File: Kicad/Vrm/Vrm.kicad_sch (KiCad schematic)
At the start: 17 parts, among them J2 Screw_Terminal_01x02, J3 Screw_Terminal_01x02, J4 AVR-JTAG-10, Q1 2N3704, SW1 Switch, U1 STM32F091RCTx

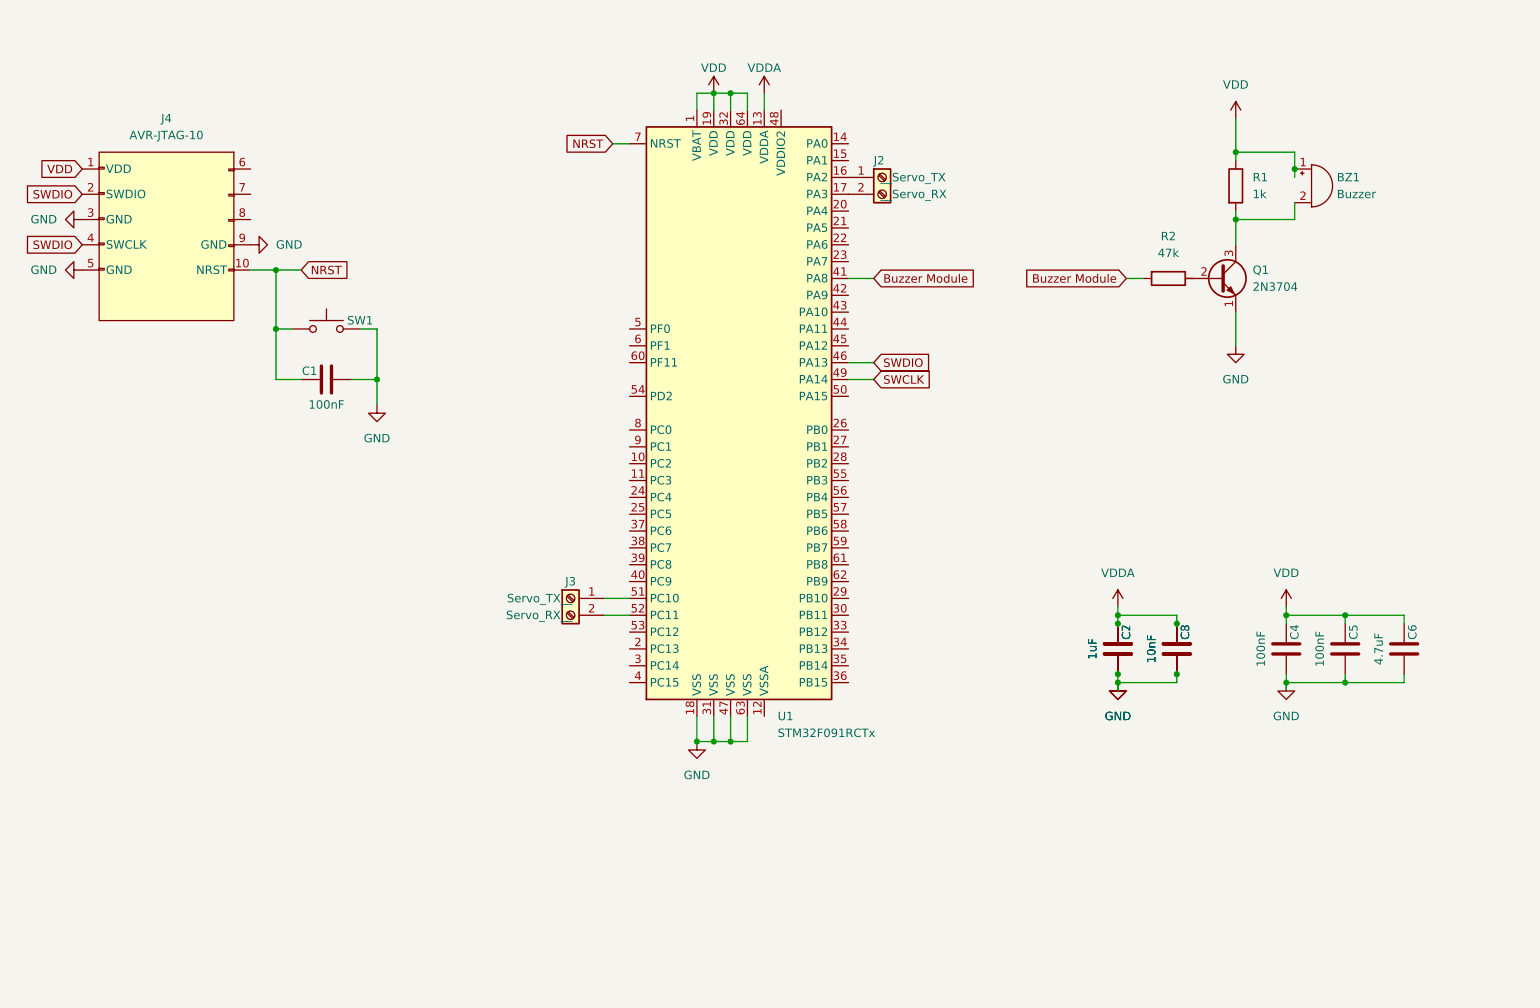
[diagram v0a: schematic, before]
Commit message: Updated schematic
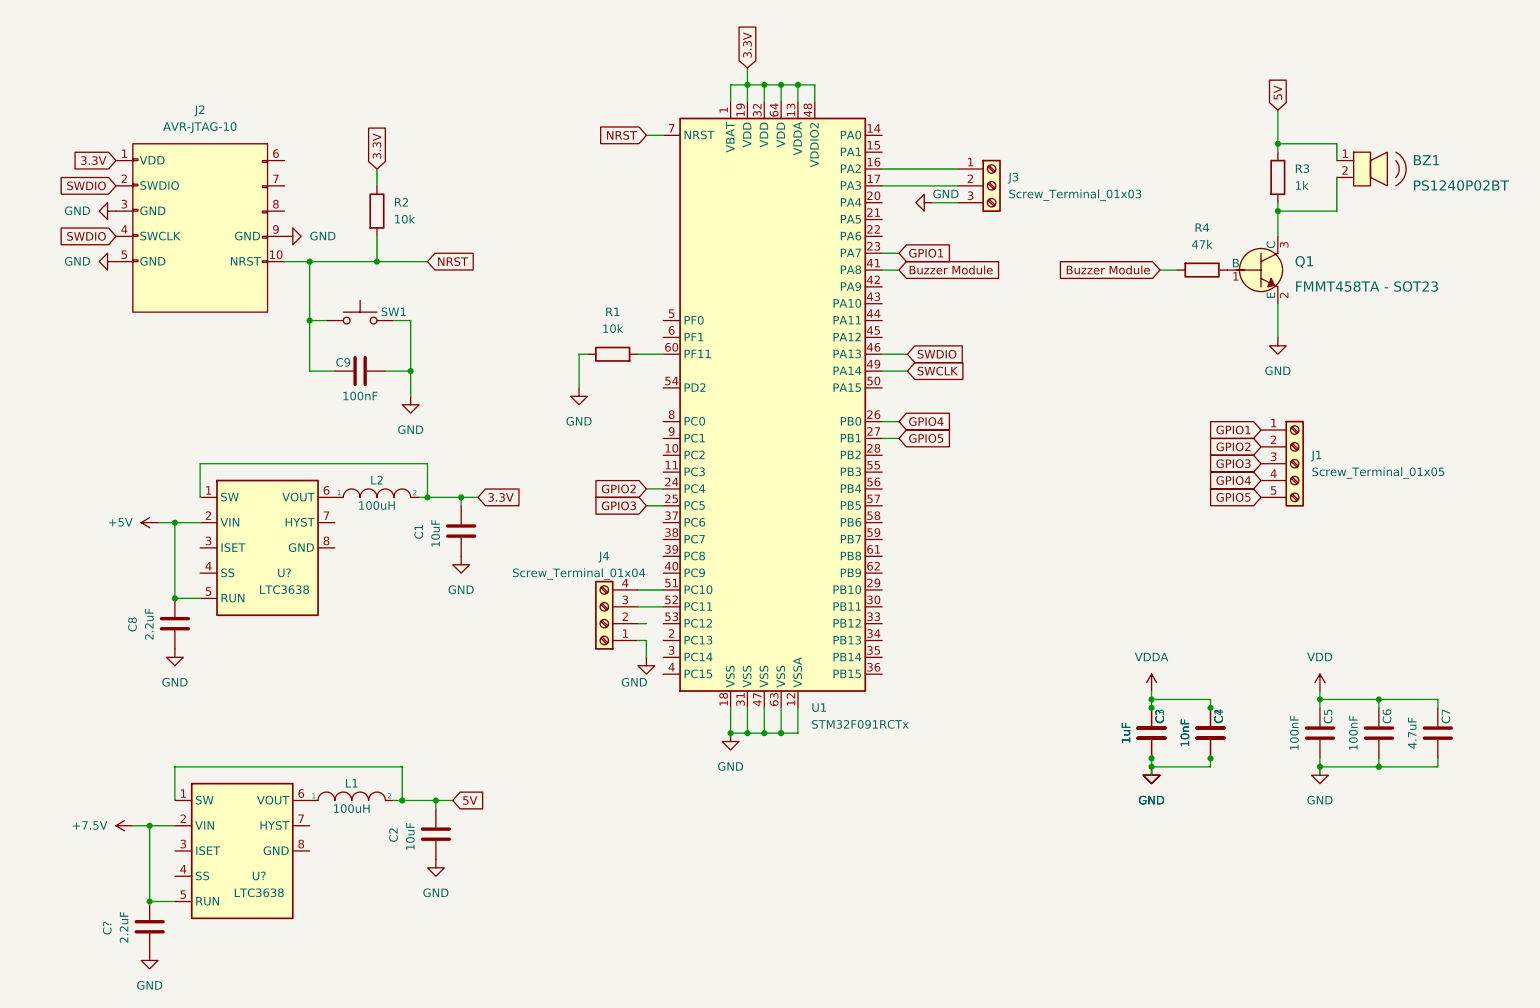
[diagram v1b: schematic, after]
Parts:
- removed BZ1: Buzzer, symbol Device:Buzzer
- removed J2, J3: Screw_Terminal_01x02, symbol Connector:Screw_Terminal_01x02
- removed J4: AVR-JTAG-10, symbol Connector:AVR-JTAG-10
- removed Q1: 2N3704, Package_TO_SOT_THT:TO-92_Inline, symbol Transistor_BJT:2N3904
- added BZ1: PS1240P02BT, digikey-footprints:Piezo_Transducer_THT_PS1240P02BT, symbol dk_Alarms-Buzzers-and-Sirens:PS1240P02BT
- added C9: 100nF, symbol Device:C
- added C?: 1uF, symbol Device:C
- added C?: 2.2uF, symbol Device:C
- added C?: 10nF, symbol Device:C
- added J1: Screw_Terminal_01x05, symbol Connector:Screw_Terminal_01x05
- added J2: AVR-JTAG-10, symbol Connector:AVR-JTAG-10
- added J3: Screw_Terminal_01x03, symbol Connector:Screw_Terminal_01x03
- added J4: Screw_Terminal_01x04, symbol Connector:Screw_Terminal_01x04
- added L1, L2: 100uH, symbol pspice:INDUCTOR
- added Q1: FMMT458TA - SOT23, digikey-footprints:SOT-23-3, symbol dk_Transistors-Bipolar-BJT-Single:FMMT458TA
- added R3: 1k, symbol Device:R
- added R4: 47k, symbol Device:R
- added U? (x2): LTC3638, Package_SO:Linear_MSOP-12-16-1EP_3x4mm_P0.5mm, symbol Regulator_Switching:LTC3638
- C1: value 100nF -> 10uF
- C2: value 1uF -> 10uF
- C3: value 10nF -> 1uF
- C4: value 100nF -> 10nF
- C6: value 4.7uF -> 100nF
- C7: value 1uF -> 4.7uF
- C8: value 10nF -> 2.2uF
- R1: value 1k -> 10k
- R2: value 47k -> 10k
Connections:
- net Buzzer Module: now also R4.2; no longer R2.2
- net GND: now also R1.1, U1.12 (VSSA), C9.2, C?.2, C?.2, C?.2, J2.3 (GND), J2.5 (GND), J2.9 (GND), J3.3 (Pin_3), J4.1 (Pin_1), Q1.2 (E)
- net NRST: now also R2.2, C9.1, J2.10 (NRST); no longer C1.1
- net SWDIO: now also J2.2 (SWDIO), J2.4 (SWCLK)
- net VDD: now also C7.1; no longer C4.1, R1.1, U1.1 (VBAT), U1.19 (VDD), U1.32 (VDD), U1.64 (VDD)
- net VDDA: now also C4.1, C?.1, C?.1; no longer C2.1, C7.1, C8.1, U1.13 (VDDA)
- net at U1.51 (PC10): now also J4.4 (Pin_4)
- net at U1.52 (PC11): now also J4.3 (Pin_3)
- net at U1.16 (PA2): now also J3.1 (Pin_1)
- net at U1.17 (PA3): now also J3.2 (Pin_2)
- net GPIO1: now reaches U1.23 (PA7)
- net GPIO1: now also J1.1 (Pin_1)
- net GPIO2: now reaches U1.24 (PC4)
- net GPIO2: now also J1.2 (Pin_2)
- net GPIO3: now reaches U1.25 (PC5)
- net GPIO3: now also J1.3 (Pin_3)
- net GPIO4: now reaches U1.26 (PB0)
- net GPIO4: now also J1.4 (Pin_4)
- net GPIO5: now reaches U1.27 (PB1)
- net GPIO5: now also J1.5 (Pin_5)
- net 3.3V: now reaches U1.48 (VDDIO2)
- net 3.3V: now also C1.1, R2.1, U1.1 (VBAT), U1.13 (VDDA), U1.19 (VDD), U1.32 (VDD), U1.64 (VDD), J2.1 (VDD), L2.2, U?.1 (SW)
- net at U1.60 (PF11): now also R1.2
- new net: L1.1, U?.6 (VOUT)
- new net: BZ1.2, Q1.3 (C), R3.2
- new net: Q1.1 (B), R4.1
- new net: L2.1, U?.6 (VOUT)
- new net +5V: C8.1, U?.2 (VIN), U?.5 (RUN)
- new net +7.5V: C?.1, U?.2 (VIN), U?.5 (RUN)
- new net 5V: BZ1.1, C2.1, L1.2, R3.1, U?.1 (SW)
